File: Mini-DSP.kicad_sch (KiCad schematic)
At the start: 95 parts, among them J1 9V, J2 Barrel_Jack_MountingPin, J3 MOBO_Con, J4 SWD, J5 USB_C_Receptacle_USB2.0_16P, SW1 USB_BOOT, SW2 USB_BOOT, SW3 MODE, U1 CS4270, U2 AMS1117-3.3, U3 W25Q128JVS, U4 AMS1117-5.0, U5 APS1604M-3SQRx-SN, U6 RP2350A-QFN60, Y1 ABM8-272-T3

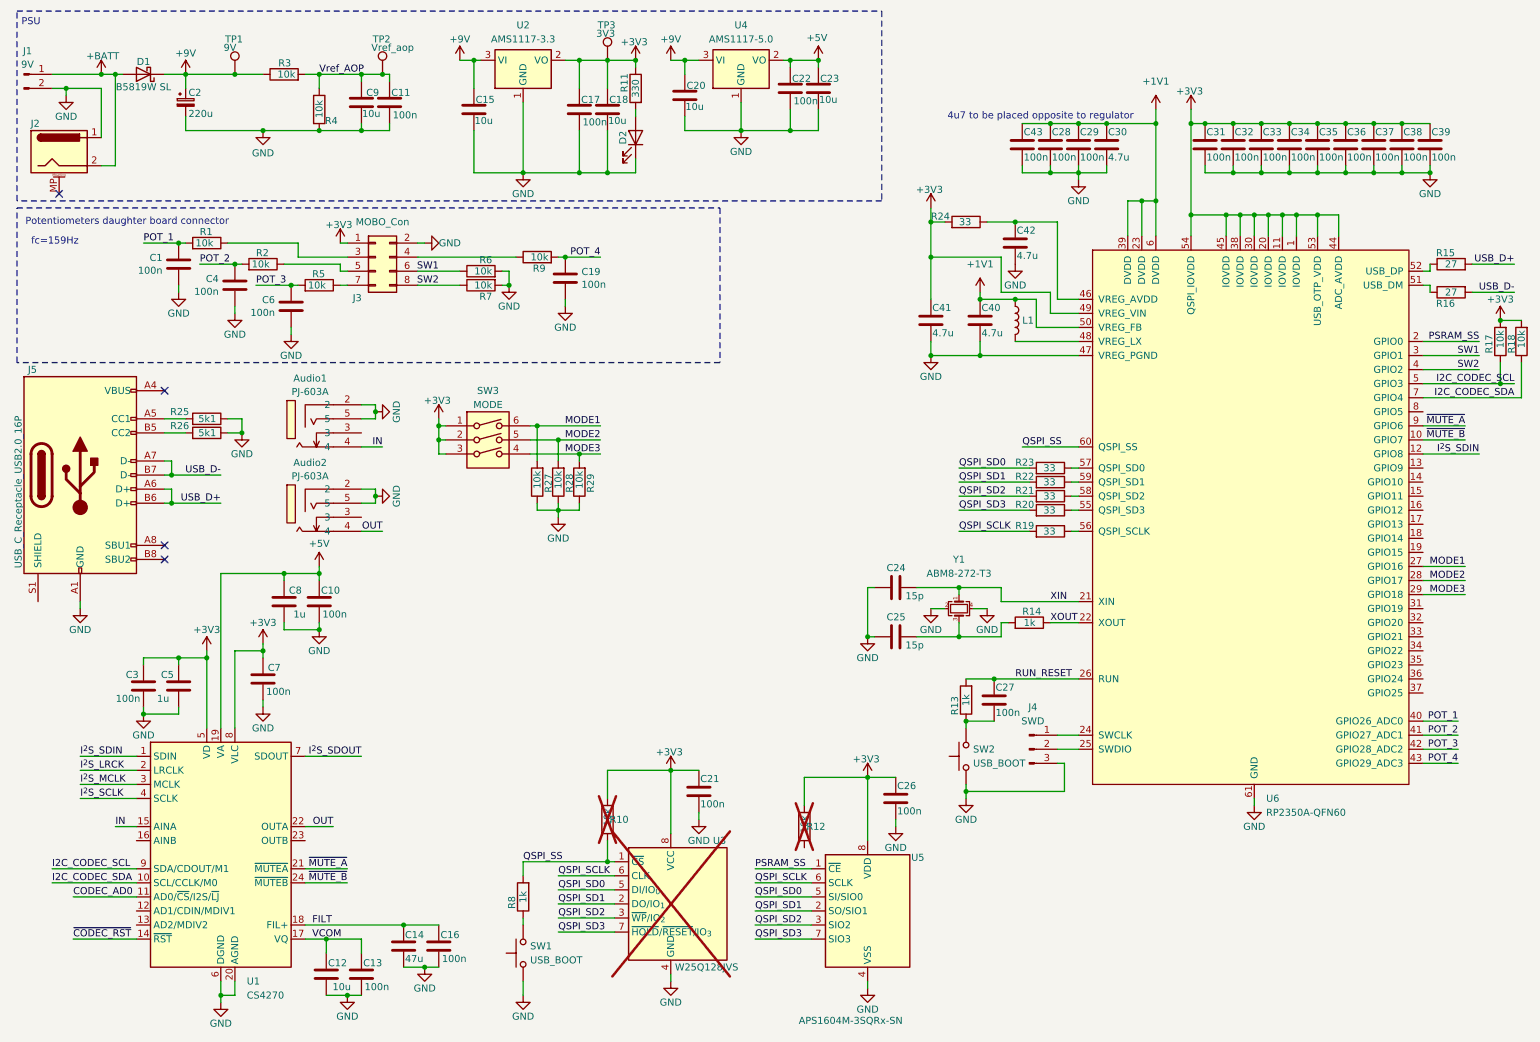
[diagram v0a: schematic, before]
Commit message: WIP
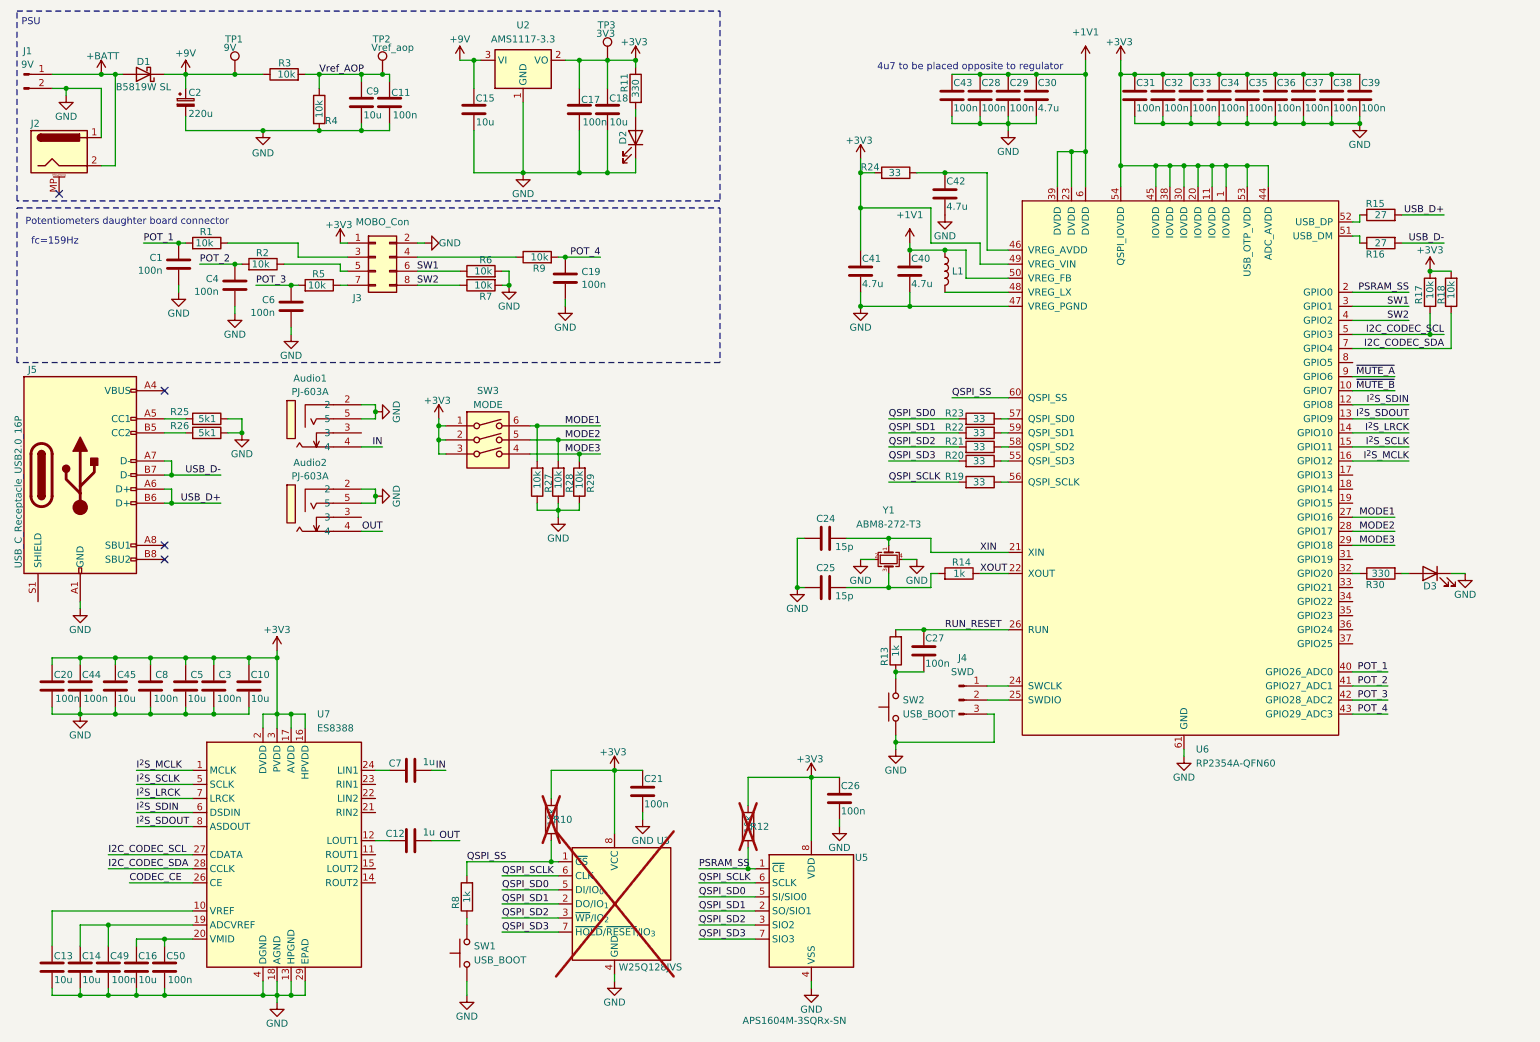
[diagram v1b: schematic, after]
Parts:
- removed C22: 100n, Capacitor_SMD:C_0402_1005Metric, symbol Device:C
- removed C23: 10u, Capacitor_SMD:C_0805_2012Metric, symbol Device:C
- removed U1: CS4270, Package_SO:TSSOP-24_4.4x7.8mm_P0.65mm, symbol Audio:CS4270
- removed U4: AMS1117-5.0, Package_TO_SOT_SMD:SOT-223-3_TabPin2, symbol Regulator_Linear:AMS1117-5.0
- added C44, C49, C50: 100n, Capacitor_SMD:C_0402_1005Metric, symbol Device:C
- added C45: 10u, Capacitor_SMD:C_0603_1608Metric, symbol Device:C
- added D3: CTL1, LED_SMD:LED_0603_1608Metric, symbol Device:LED
- added R30: 330, Resistor_SMD:R_0402_1005Metric, symbol Device:R
- added U7: ES8388, Package_DFN_QFN:QFN-28-1EP_4x4mm_P0.45mm_EP2.6x2.6mm, symbol Audio:ES8388
- C10, C13, C16: value 100n -> 10u; footprint Capacitor_SMD:C_0402_1005Metric -> Capacitor_SMD:C_0603_1608Metric
- C12: value 10u -> 1u
- C14: value 47u -> 10u; footprint Capacitor_SMD:C_1206_3216Metric -> Capacitor_SMD:C_0603_1608Metric
- C15, C18, C9: footprint Capacitor_SMD:C_0805_2012Metric -> Capacitor_SMD:C_0603_1608Metric
- C20: value 10u -> 100n; footprint Capacitor_SMD:C_0805_2012Metric -> Capacitor_SMD:C_0402_1005Metric
- C5: value 1u -> 10u; footprint Capacitor_SMD:C_0805_2012Metric -> Capacitor_SMD:C_0603_1608Metric
- C7: value 100n -> 1u; footprint Capacitor_SMD:C_0402_1005Metric -> Capacitor_SMD:C_0805_2012Metric
- C8: value 1u -> 100n; footprint Capacitor_SMD:C_0805_2012Metric -> Capacitor_SMD:C_0402_1005Metric
- U6: value RP2350A-QFN60 -> RP2354A-QFN60
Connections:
- net +5V is gone; now on net +3V3: C10.1, C8.1
- net +3V3: now also C20.1, C44.1, C45.1, U7.16 (HPVDD), U7.17 (AVDD), U7.2 (DVDD), U7.3 (PVDD); no longer C7.1
- net +9V: no longer C20.1
- net GND: now also C44.2, C45.2, C49.2, C50.2, D3.1 (K), U7.13 (HPGND), U7.18 (AGND), U7.29 (EPAD), U7.4 (DGND); no longer C12.2, C7.2
- net I2C_CODEC_SCL: now also U7.27 (CDATA)
- net I2C_CODEC_SDA: now also U7.28 (CCLK)
- net IN: now also C7.2
- net I^{2}S_LRCK: now also U6.14 (GPIO10), U7.7 (LRCK)
- net I^{2}S_MCLK: now also U6.16 (GPIO12), U7.1 (MCLK)
- net I^{2}S_SCLK: now also U6.15 (GPIO11), U7.5 (SCLK)
- net I^{2}S_SDIN: now also U7.6 (DSDIN)
- net I^{2}S_SDOUT: now also U6.13 (GPIO9), U7.8 (ASDOUT)
- net OUT: now also C12.2
- net PSRAM_SS: now also R12.1
- net at U6.32 (GPIO20): now also R30.1
- net FILT: no longer names the net of C14.1
- net FILT: now also C49.1, U7.19 (ADCVREF); no longer C16.1
- net VCOM: no longer names the net of C12.1
- net VCOM: now also U7.12 (LOUT1); no longer C13.1
- new net: C13.1, U7.10 (VREF)
- new net: C16.1, C50.1, U7.20 (VMID)
- new net: C7.1, U7.24 (LIN1)
- new net: D3.2 (A), R30.2
- new net CODEC_CE: U7.26 (CE)
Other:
- moved on the sheet: C21, C24, C25, C26, C27, C28, C29, C3, C30, C31, C32, C33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
